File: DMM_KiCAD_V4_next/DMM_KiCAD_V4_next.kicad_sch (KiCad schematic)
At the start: 70 parts, among them J1 Conn_01x07_Pin, J11 I_Input, J12 Conn_01x02_Pin, J14 Barrel_Jack, J15 Barrel_Jack, J16 Conn_01x01_Socket, J17 Conn_01x01_Socket, J2 MicoSD, J3 Conn_01x07_Pin, J7 Conn_01x02_Pin, J9 Out to Screen, Q1 MMBT3904, Q2 AO3400A, Q6 BSS138, Q7 BSS138, Q8 AO3400A MOSFET, SW1 SW_Push, SW2 SW_Push, SW3 SW_SPDT, SW4 SW_Push, U1 LM317_TO-220, U10 LM4040DBZ-2.5, U11 LM4040DBZ-5, U2 IX4426N, U3 ADS1115IDGS, U4 IX4426N, U5 TLV61046ADBVR, U7 MAX1683, U9 TPS613222ADBV

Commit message: Minor KiCAD updates and file reorganization
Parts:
- removed A1: Arduino_Nano_ESP32, Module:Arduino_Nano, symbol MCU_Module:Arduino_Nano_ESP32
- removed U5: TLV61046ADBVR, Package_TO_SOT_SMD:SOT-23-6_Handsoldering, symbol CustomLibrary:TLV61046ADBVR
- added J10: ANALOG, Library:PinHeader_1x06_P2.54mm_Vertical_NoBox, symbol Connector_Generic:Conn_01x06
- added J13: DIGITAL1, Library:PinHeader_1x08_P2.54mm_Vertical_NoBox, symbol Connector_Generic:Conn_01x08
- added J5: POWER2, Library:PinHeader_1x03_P2.54mm_Vertical_NoBox, symbol Connector_Generic:Conn_01x03
- added J6: POWER1, Library:PinHeader_1x08_P2.54mm_Vertical_NoBox, symbol Connector_Generic:Conn_01x08
- added J8: DIGITAL2, Library:PinHeader_1x10_P2.54mm_Vertical_NoBox, symbol Connector_Generic:Conn_01x10
- added R11, R19, R20: 10K, Resistor_SMD:R_0805_2012Metric_Pad1.20x1.40mm_HandSolder, symbol Device:R_US
- added R22: 0, Resistor_SMD:R_0805_2012Metric_Pad1.20x1.40mm_HandSolder, symbol Device:R_US
- added R8: 71.5k, Resistor_SMD:R_0805_2012Metric_Pad1.20x1.40mm_HandSolder, symbol Device:R_US
- added U12: TLV61046ADBVR, Package_TO_SOT_SMD:SOT-23-6_Handsoldering, symbol CustomLibrary:TLV61046ADBVR
- added U5, U8: Opamp_Dual, Package_SO:SOIC-8_3.9x4.9mm_P1.27mm, symbol Device:Opamp_Dual
- Q2: value AO3400A -> AO3400A MOSFET
- R10: value 71.5k -> 10K; now not fitted
- R14: value 22.0K -> 15.0K
- RN1, RN2: footprint Library:RESCAXS127P508X320X70-8N -> Resistor_SMD:R_Array_Convex_4x1206
- renumbered R8 to R25
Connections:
- net +3V3: now also J6.4 (Pin_4)
- net +9V: now also U12.5 (VOUT)
- net +VSW: now also J6.8 (Pin_8)
- net A0/D14: now also J10.1 (Pin_1)
- net A1/D15: now also J10.2 (Pin_2)
- net A2/D16: now also J10.3 (Pin_3)
- net A3/D17: now also J10.4 (Pin_4)
- net ADC-1: now also Q8.2 (S); no longer R24.1
- net CLK: now also J8.6 (Pin_6)
- net CS: now also J8.3 (Pin_3)
- net D10~: now also J13.5 (Pin_5)
- net D3~: now also J13.4 (Pin_4)
- net D5~ (IR): now also J13.6 (Pin_6)
- net D6~: now also J13.7 (Pin_7)
- net D7: now also J13.8 (Pin_8)
- net D9~: now also J13.3 (Pin_3)
- net GND: now also J5.2 (Pin_2), J6.6 (Pin_6), J6.7 (Pin_7), J8.7 (Pin_7), R8.2, U12.2 (GND); no longer R10.2
- net MISO: now also J8.5 (Pin_5)
- net MOSI: now also J8.4 (Pin_4)
- net SCL: now also J8.10 (Pin_10)
- net SCL-5V: now also RN1.3 (R3.1); no longer RN1.2 (R4.1)
- net SDA: now also J8.9 (Pin_9)
- net SDA-5V: now also RN1.2 (R4.1); no longer RN1.3 (R3.1)
- net Uno5vPin: now also J6.5 (Pin_5), R22.2
- net V Ref to ADS-0: now also R14.1; no longer Q8.3 (D)
- net VDD: now also R22.1, U12.6 (VIN)
- net at C1.1, C5.1, C6.1: now also U12.4 (EN)
- net at R25.2: now also R8.1, U12.3 (FB); no longer R10.1
- net at L2.2: now also U12.1 (SW)
- new net: Q8.3 (D), R24.1
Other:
- company: (none) -> Nick Mann
- title: (none) -> Arduino Uno DMM Shield
- moved on the sheet: C1, C10, C15, C16, C17, C18, C19, C2, C3, C4, C5, C6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

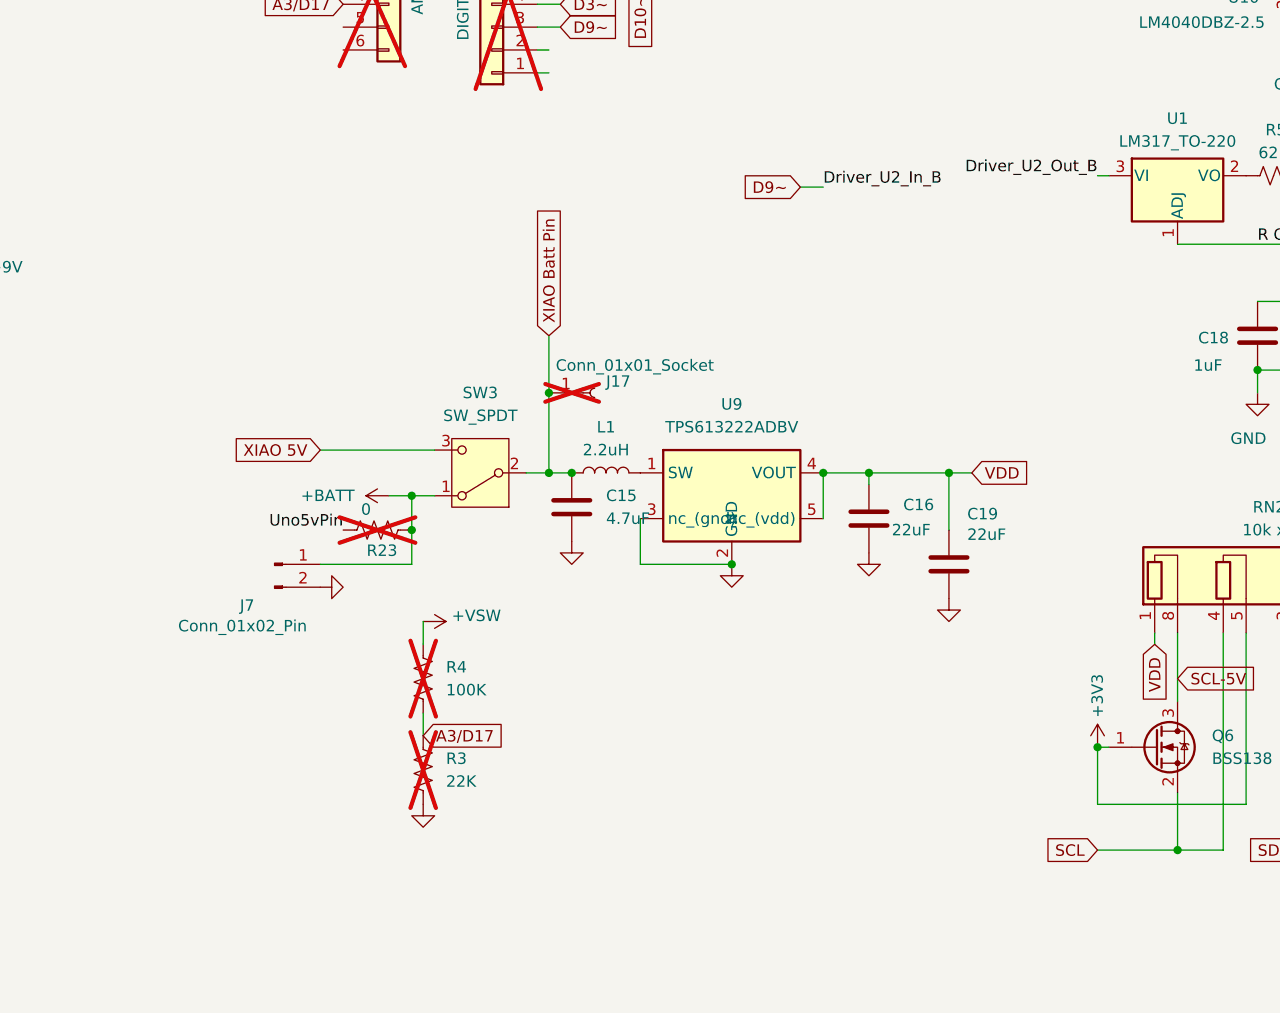
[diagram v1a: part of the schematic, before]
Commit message: Working on the next PCBs
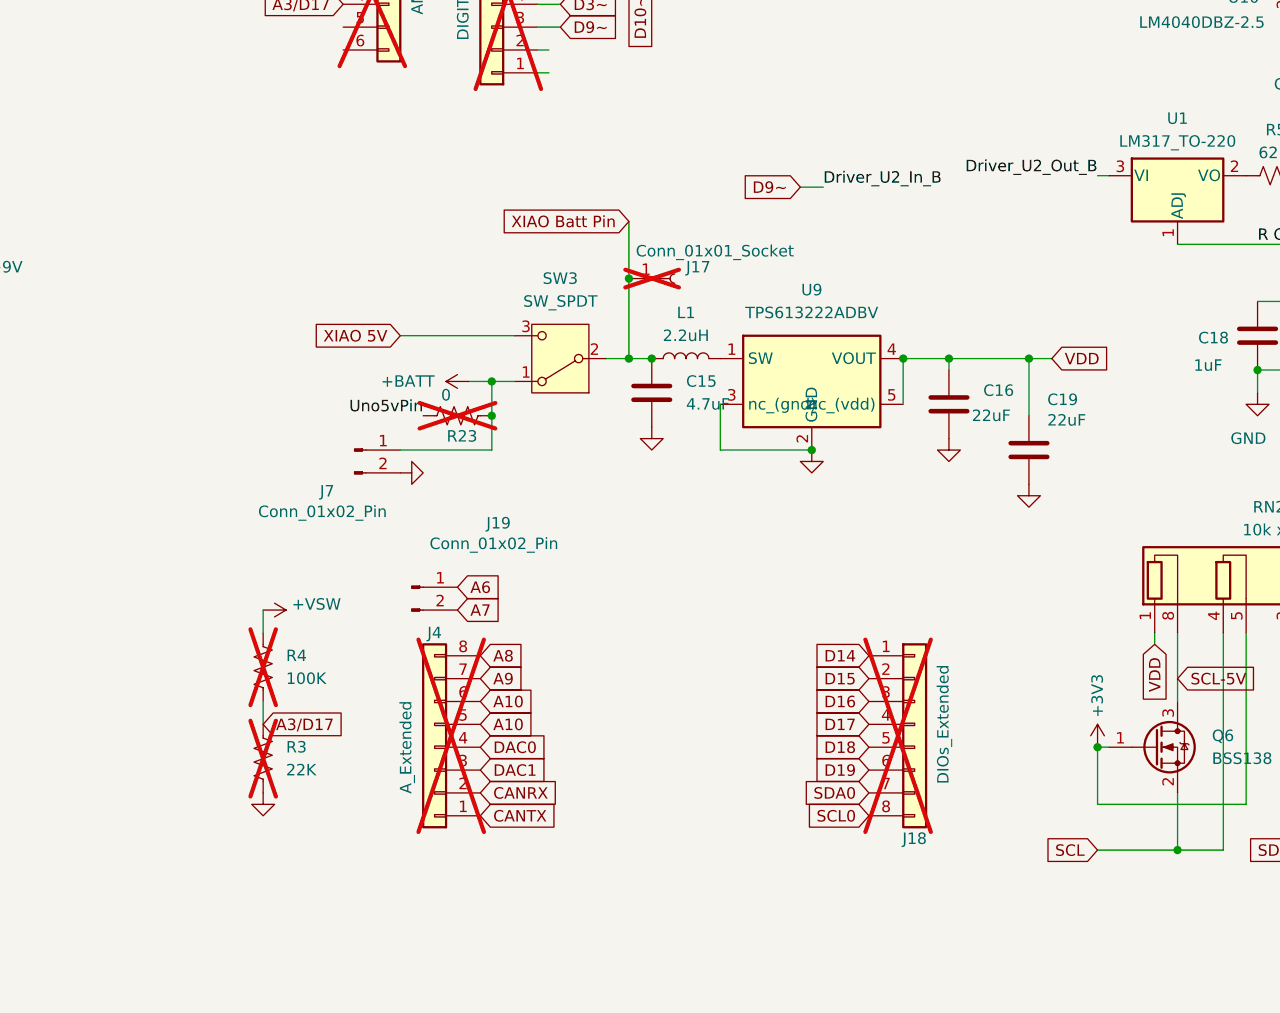
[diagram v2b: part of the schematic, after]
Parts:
- added J18: DIOs_Extended, Connector_PinHeader_2.54mm:PinHeader_1x08_P2.54mm_Vertical, symbol Connector_Generic:Conn_01x08
- added J19: Conn_01x02_Pin, Connector_PinSocket_2.54mm:PinSocket_1x02_P2.54mm_Vertical, symbol Connector:Conn_01x02_Pin
- added J4: A_Extended, Connector_PinHeader_2.54mm:PinHeader_1x08_P2.54mm_Vertical, symbol Connector_Generic:Conn_01x08
- RN1, RN2: footprint Resistor_SMD:R_Array_Convex_4x1206 -> Library:RESCAXS127P508X320X70-8N
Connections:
- new net A10: J4.5 (Pin_5), J4.6 (Pin_6)
- new net A6: J19.1 (Pin_1)
- new net A7: J19.2 (Pin_2)
- new net A8: J4.8 (Pin_8)
- new net A9: J4.7 (Pin_7)
- new net CANRX: J4.2 (Pin_2)
- new net CANTX: J4.1 (Pin_1)
- new net D14: J18.1 (Pin_1)
- new net D15: J18.2 (Pin_2)
- new net D16: J18.3 (Pin_3)
- new net D17: J18.4 (Pin_4)
- new net D18: J18.5 (Pin_5)
- new net D19: J18.6 (Pin_6)
- new net DAC0: J4.4 (Pin_4)
- new net DAC1: J4.3 (Pin_3)
- new net SCL0: J18.8 (Pin_8)
- new net SDA0: J18.7 (Pin_7)
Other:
- moved on the sheet: C15, C16, C19, J17, J7, L1, R23, R3, R4, SW3, U9
